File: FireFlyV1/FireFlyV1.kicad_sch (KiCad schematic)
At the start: 59 parts, among them J1 Conn_01x03, J2 Conn_01x01_Pin, J3 Conn_01x01_Pin, SW1 TS-1187A-B-A-B, SW2 TS-1187A-B-A-B, U1 RP2040, U2 W25Q32JVSS, U3 AMS1117-3.3, U5 MCP6001T-I/OT, U7 PEC12R-4215F-S0024, X1 X322512MSB4SI

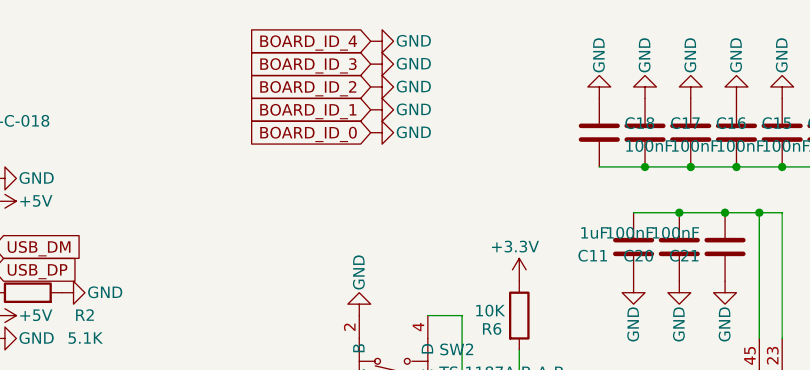
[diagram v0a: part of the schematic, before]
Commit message: Questionable routing decisions
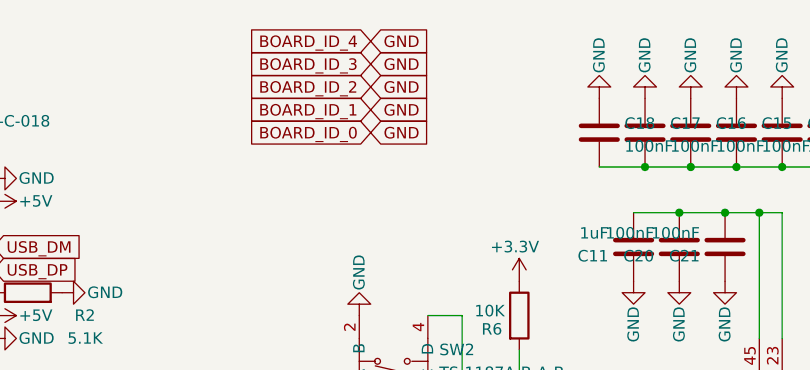
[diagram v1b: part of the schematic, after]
